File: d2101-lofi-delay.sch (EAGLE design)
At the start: 65 parts, among them U3 FX2-20P-1.27DS, U4 FX2-20S-1.27DS

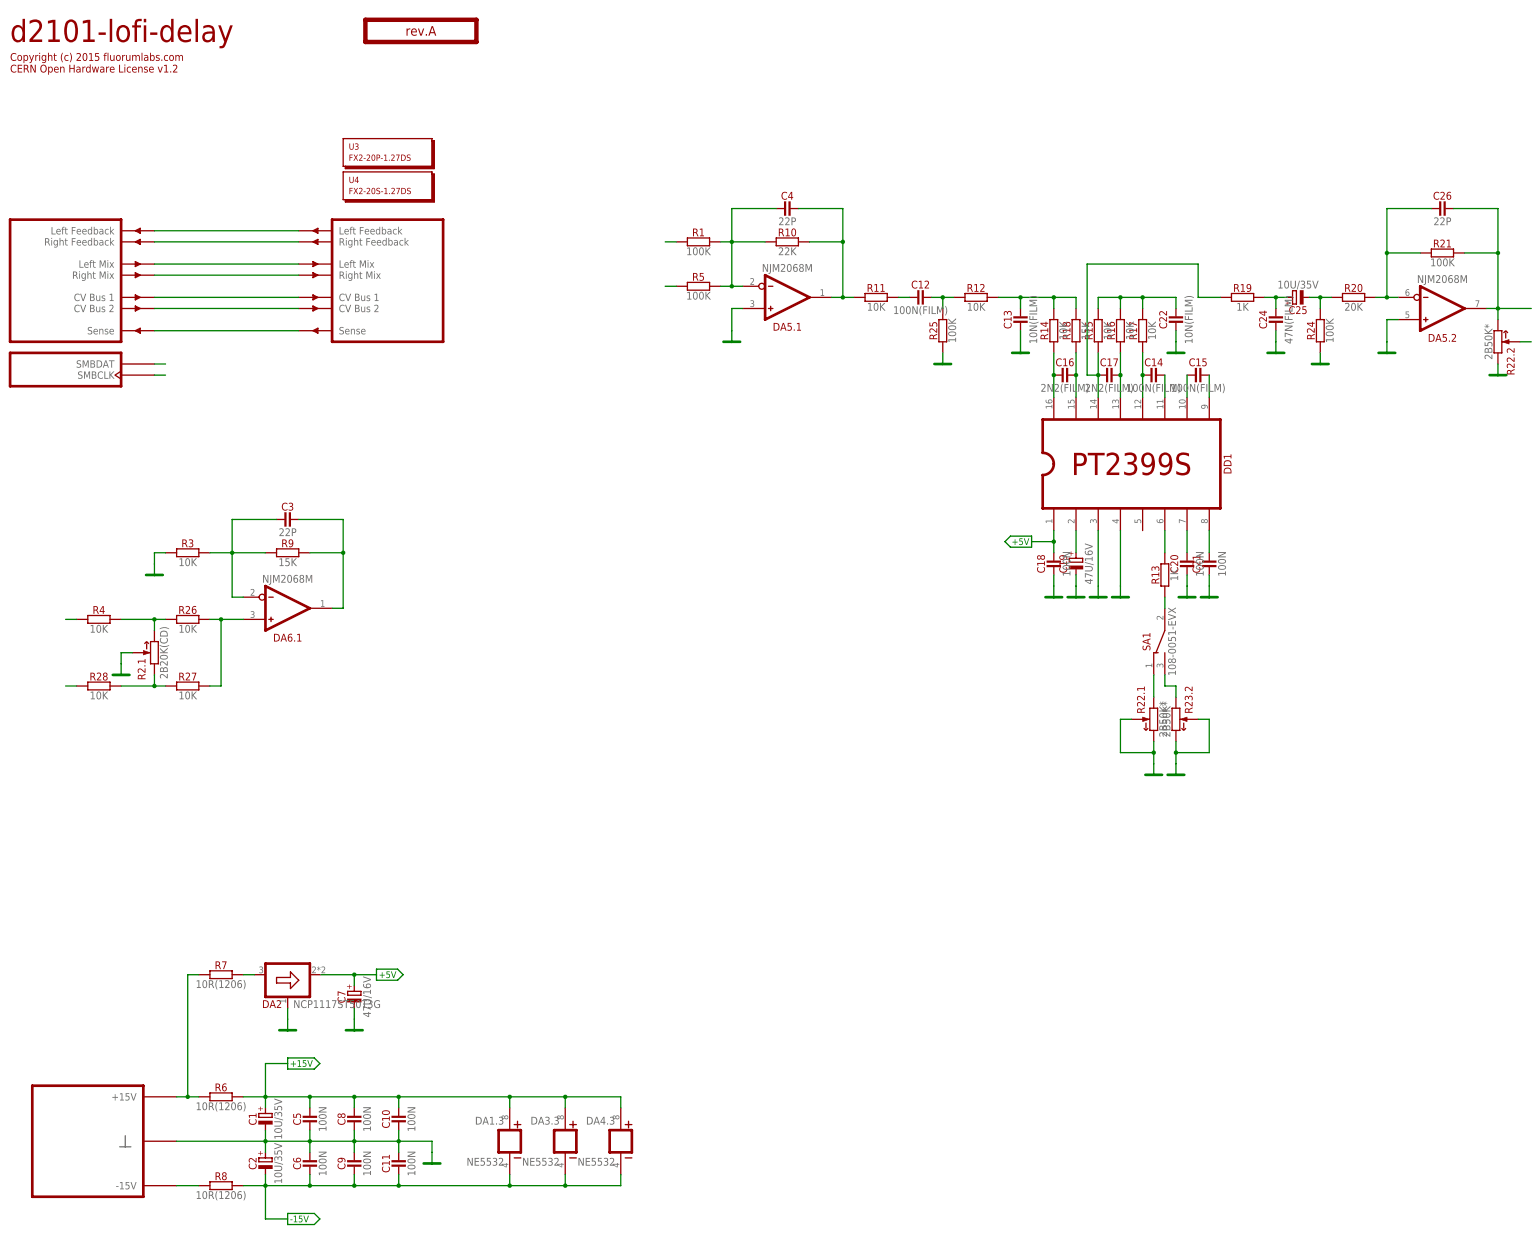
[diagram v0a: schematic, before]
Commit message: D2101 done
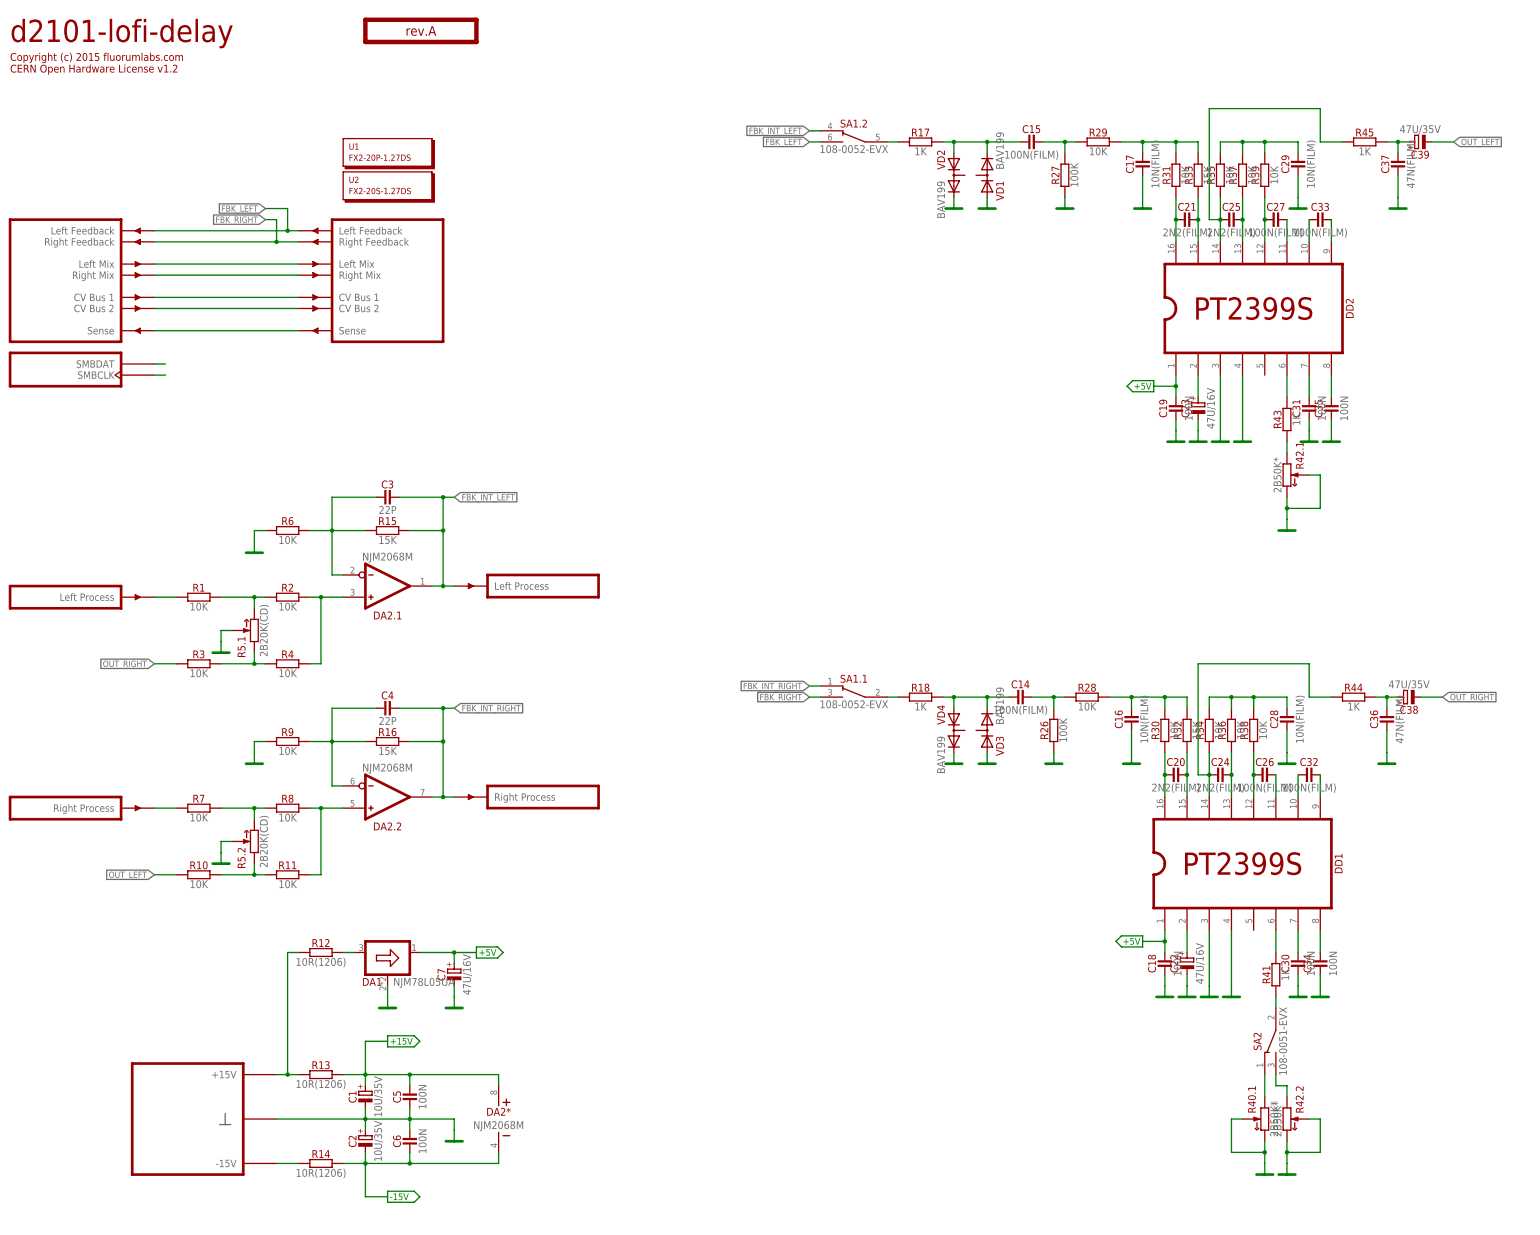
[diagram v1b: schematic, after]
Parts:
- removed C10, C11, C8, C9: 100N, capacitors:100N
- removed C12: 100N(FILM), capacitors:100N(FILM)
- removed C13: 10N(FILM), capacitors:10N(FILM)
- removed DA3, DA4: NE5532, f-opamp:OPAMP-DUAL-SO
- removed DA5, DA6: NJM2068M, ic-jrc:NJM2068M
- removed R19: 1K, resistors:1K
- removed R20: 20K, resistors:20K
- removed R21, R24, R25: 100K, resistors:100K
- removed R22, R23: 2B50K*, potentiometers:2B50K*
- added C23: 47U/16V, capacitors-electrolytic:47U/16V
- added C27, C32, C33: 100N(FILM), capacitors:100N(FILM)
- added C28, C29: 10N(FILM), capacitors:10N(FILM)
- added C30, C31, C34, C35: 100N, capacitors:100N
- added C36, C37: 47N(FILM), capacitors:47N(FILM)
- added C38, C39: 47U/35V, capacitors-electrolytic:47U/35V
- added DD2: PT2399S, ic-princeton-technologies:PT2399S
- added R29, R30, R31, R34, R35, R36, R37, R38, R39: 10K, resistors:10K
- added R32, R33: 15K, resistors:15K
- added R40, R42: 2B50K*, potentiometers:2B50K*
- added R41, R43, R44, R45: 1K, resistors:1K
- added SA2: 108-0051-EVX, switches:108-0051-EVX
- added VD1, VD2, VD3, VD4: BAV199, diodes:BAV199
- C16, C17: value 2N2(FILM) -> 10N(FILM); device capacitors:2N2(FILM) -> capacitors:10N(FILM)
- C19: value 47U/16V -> 100N; device capacitors-electrolytic:47U/16V -> capacitors:100N
- C20, C21: value 100N -> 2N2(FILM); device capacitors:100N -> capacitors:2N2(FILM)
- C22: value 10N(FILM) -> 47U/16V; device capacitors:10N(FILM) -> capacitors-electrolytic:47U/16V
- C24: value 47N(FILM) -> 2N2(FILM); device capacitors:47N(FILM) -> capacitors:2N2(FILM)
- C25: value 10U/35V -> 2N2(FILM); device capacitors-electrolytic:10U/35V -> capacitors:2N2(FILM)
- C26: value 22P -> 100N(FILM); device capacitors:22P -> capacitors:100N(FILM)
- DA1: value NE5532 -> NJM78L05UA; device f-opamp:OPAMP-DUAL-SO -> regulators-linear:NJM78L05UA; PARTNO OP275GSZ -> (none)
- DA2: value NCP1117ST50T3G -> NJM2068M; device regulators-linear:NCP1117ST50T3G -> ic-jrc:NJM2068M
- R1: value 100K -> 10K; device resistors:100K -> resistors:10K
- R10: value 22K -> 10K; device resistors:22K -> resistors:10K
- R12, R14: value 10K -> 10R(1206); device resistors:10K -> resistors:10R(1206)
- R13: value 1K -> 10R(1206); device resistors:1K -> resistors:10R(1206)
- R15, R16: value 10K -> 15K; device resistors:10K -> resistors:15K
- R17: value 10K -> 1K; device resistors:10K -> resistors:1K
- R18: value 15K -> 1K; device resistors:15K -> resistors:1K
- R2: value 2B20K(CD) -> 10K; device potentiometers:2B20K(CD) -> resistors:10K
- R26, R27: value 10K -> 100K; device resistors:10K -> resistors:100K
- R5: value 100K -> 2B20K(CD); device resistors:100K -> potentiometers:2B20K(CD)
- R6, R7, R8: value 10R(1206) -> 10K; device resistors:10R(1206) -> resistors:10K
- R9: value 15K -> 10K; device resistors:15K -> resistors:10K
- SA1: value 108-0051-EVX -> 108-0052-EVX; device switches:108-0051-EVX -> switches:108-0052-EVX
- renumbered U3 to U1, U4 to U2
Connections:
- removed net N$12: C25.-, R20.1, R24.2
- removed net N$26: R1.1
- removed net N$27: R22.2.W
- removed net N$29: C3.2, DA6.1.OUT, R9.2
- removed net N$66: R13.1, SA1.CM
- new net FBK_INT_LEFT: C3.2, DA2.1.OUT, PCB1G$4.OUTL, R15.2, SA1.2.NC
- new net FBK_INT_RIGHT: C4.2, DA2.2.OUT, PCB1G$5.OUTR, R16.2, SA1.1.NC
- new net FBK_LEFT: PCB1G$6.LFBK, PCB1G$7.LFBK', SA1.2.NO
- new net FBK_RIGHT: PCB1G$6.RFBK, PCB1G$7.RFBK', SA1.1.NO
- new net N$39: DA2.2.IN+, R11.2, R8.2
- new net N$40: R10.2, R11.1, R5.2.CCW
- new net N$48: C28.2, R34.2, R36.2, R38.2
- new net N$49: C20.1, DD1.16, R30.1
- new net N$50: C20.2, DD1.15, R32.1
- new net N$51: C24.1, DD1.14, R34.1, R44.1
- new net N$52: C24.2, DD1.13, R36.1
- new net N$53: C26.1, DD1.12, R38.1
- new net N$54: C26.2, DD1.11
- new net N$55: C32.1, DD1.10
- new net N$56: C32.2, DD1.9
- new net N$57: C36.2, C38.+, R44.2
- new net N$58: C30.2, DD1.7
- new net N$59: C34.2, DD1.8
- new net N$60: DD1.6, R41.2
- new net N$62: C14.2, R26.2, R28.1
- new net N$63: C16.2, R28.2, R30.2, R32.2
- new net N$69: C22.+, DD1.2
- new net OUT_LEFT: C39.-, R10.1
- new net OUT_RIGHT: C38.-, R3.1
- net +15V: now also DA2*.V+, R13.2; no longer C10.2, C8.2, DA1.3.V+15, DA3.3.V+15, DA4.3.V+15, R6.2
- net +5V: now also C19.2, DA1.OUT, DD2.1; no longer DA2.OUT
- net -15V: now also DA2*.V-, R14.2; no longer C11.1, C9.1, DA1.3.V-15, DA3.3.V-15, DA4.3.V-15, R8.2
- net GND: now also C16.1, C17.1, C19.1, C22.-, C23.-, C28.1, C29.1, C30.1, C31.1, C34.1, C35.1, C36.1, C37.1, DA1.GND, DD2.3, DD2.4, R26.1, R27.1, R40.1.CW, R40.1.W, R42.1.CW, R42.1.W, R42.2.CW, R42.2.W, R5.1.W, R5.2.W, R6.1, R9.1, VD1.A, VD2.C, VD3.A, VD4.C; no longer C10.1, C11.2, C13.1, C19.-, C20.1, C21.1, C22.1, C24.1, C8.1, C9.2, DA2.GND, DA5.1.IN+, DA5.2.IN+, R2.1.W, R22.1.CW, R22.1.W, R22.2.CCW, R23.2.CW, R23.2.W, R24.1, R25.1, R3.1
- net N$1: now also R42.1.CCW, R43.1; no longer PCB1G$6.LFBK, PCB1G$7.LFBK'
- net N$10: now also C17.2, R29.2, R31.2, R33.2; no longer C13.2, R12.2, R14.2, R18.2
- net N$11: now also PCB1G$2.INL, R1.1; no longer R28.1
- net N$13: now also R18.1, SA1.1.CM; no longer C26.1, DA5.2.IN-, R20.2, R21.1
- net N$14: now also R42.2.CCW, SA2.NO; no longer R23.2.CCW, SA1.NO
- net N$15: now also C29.2, R35.2, R37.2, R39.2; no longer C22.2, R15.2, R16.2, R17.2
- net N$17: now also C21.2, DD2.15, R33.1; no longer C16.2, DD1.15, R18.1
- net N$18: now also C25.1, DD2.14, R35.1, R45.1; no longer C17.1, DD1.14, R15.1, R19.1
- net N$19: now also C25.2, DD2.13, R37.1; no longer C17.2, DD1.13, R16.1
- net N$2: now also R41.1, SA2.CM; no longer PCB1G$6.RFBK, PCB1G$7.RFBK'
- net N$20: now also C27.1, DD2.12, R39.1; no longer C14.1, DD1.12, R17.1
- net N$21: now also C27.2, DD2.11; no longer C14.2, DD1.11
- net N$22: now also C33.1, DD2.10; no longer C15.1, DD1.10
- net N$23: now also C33.2, DD2.9; no longer C15.2, DD1.9
- net N$24: now also C37.2, C39.+, R45.2; no longer C24.2, C25.+, R19.2
- net N$25: now also C4.1, DA2.2.IN-, R16.1, R9.2; no longer R5.1
- net N$28: now also PCB1G$3.INR, R7.1; no longer R4.1
- net N$3: now also C15.1, R17.2, VD1.C, VD2.A; no longer C4.1, DA5.1.IN-, R1.2, R10.1, R5.2
- net N$30: now also R1.2, R2.1, R5.1.CW; no longer R2.1.CW, R26.1, R4.2
- net N$31: now also C31.2, DD2.7; no longer C20.2, DD1.7
- net N$32: now also C35.2, DD2.8; no longer C21.2, DD1.8
- net N$33: now also DD2.6, R43.2; no longer DD1.6, R13.2
- net N$36: now also R14.1; no longer R8.1
- net N$37: now also C23.+, DD2.2; no longer C19.+, DD1.2
- net N$4: now also C21.1, DD2.16, R31.1; no longer C16.1, DD1.16, R14.1
- net N$44: now also DA1.IN, R12.2; no longer DA2.IN, R7.2
- net N$5: now also C14.1, R18.2, VD3.C, VD4.A; no longer C4.2, DA5.1.OUT, R10.2, R11.1
- net N$6: now also R17.1, SA1.2.CM; no longer C12.1, R11.2
- net N$61: now also DA2.1.IN+, R2.2, R4.2; no longer DA6.1.IN+, R26.2, R27.2
- net N$64: now also DA2.1.IN-, R15.1, R6.2; no longer DA6.1.IN-, R3.2, R9.1
- net N$65: now also R3.2, R4.1, R5.1.CCW; no longer R2.1.CCW, R27.1, R28.2
- net N$7: now also R5.2.CW, R7.2, R8.1; no longer C26.2, DA5.2.OUT, R21.2, R22.2.CW
- net N$8: now also R40.1.CCW, SA2.NC; no longer R22.1.CCW, SA1.NC
- net N$9: now also C15.2, R27.2, R29.1; no longer C12.2, R12.1, R25.2
- net P+15V: now also R12.1, R13.1; no longer R6.1, R7.1
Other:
- moved on the sheet: C1, C14, C15, C16, C17, C18, C2, C20, C21, C24, C26, C3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
